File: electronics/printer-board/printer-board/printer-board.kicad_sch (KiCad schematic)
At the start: 38 parts, among them J1 XM, J10 THE1, J11 FAN1, J12 ZM1, J13 HE2, J14 THE2, J15 FAN2, J16 TFT, J17 EXP2, J18 EM0, J19 E0-Stop, J2 NeoPixel, J20 X-Stop, J21 EM1, J22 E1-Stop, J23 Y-Stop, J24 Bed, J25 I2C, J26 EM2, J27 E2-Stop, J28 Z-Stop, J29 Bed, J3 THB, J30 Hotend, J32 5V_PSU, J33 Hotend, J35 Extension1, J36 Extension2, J4 EXP1, J5 YM, J6 THE0, J7 FAN0, J8 BLTouch, J9 HE1

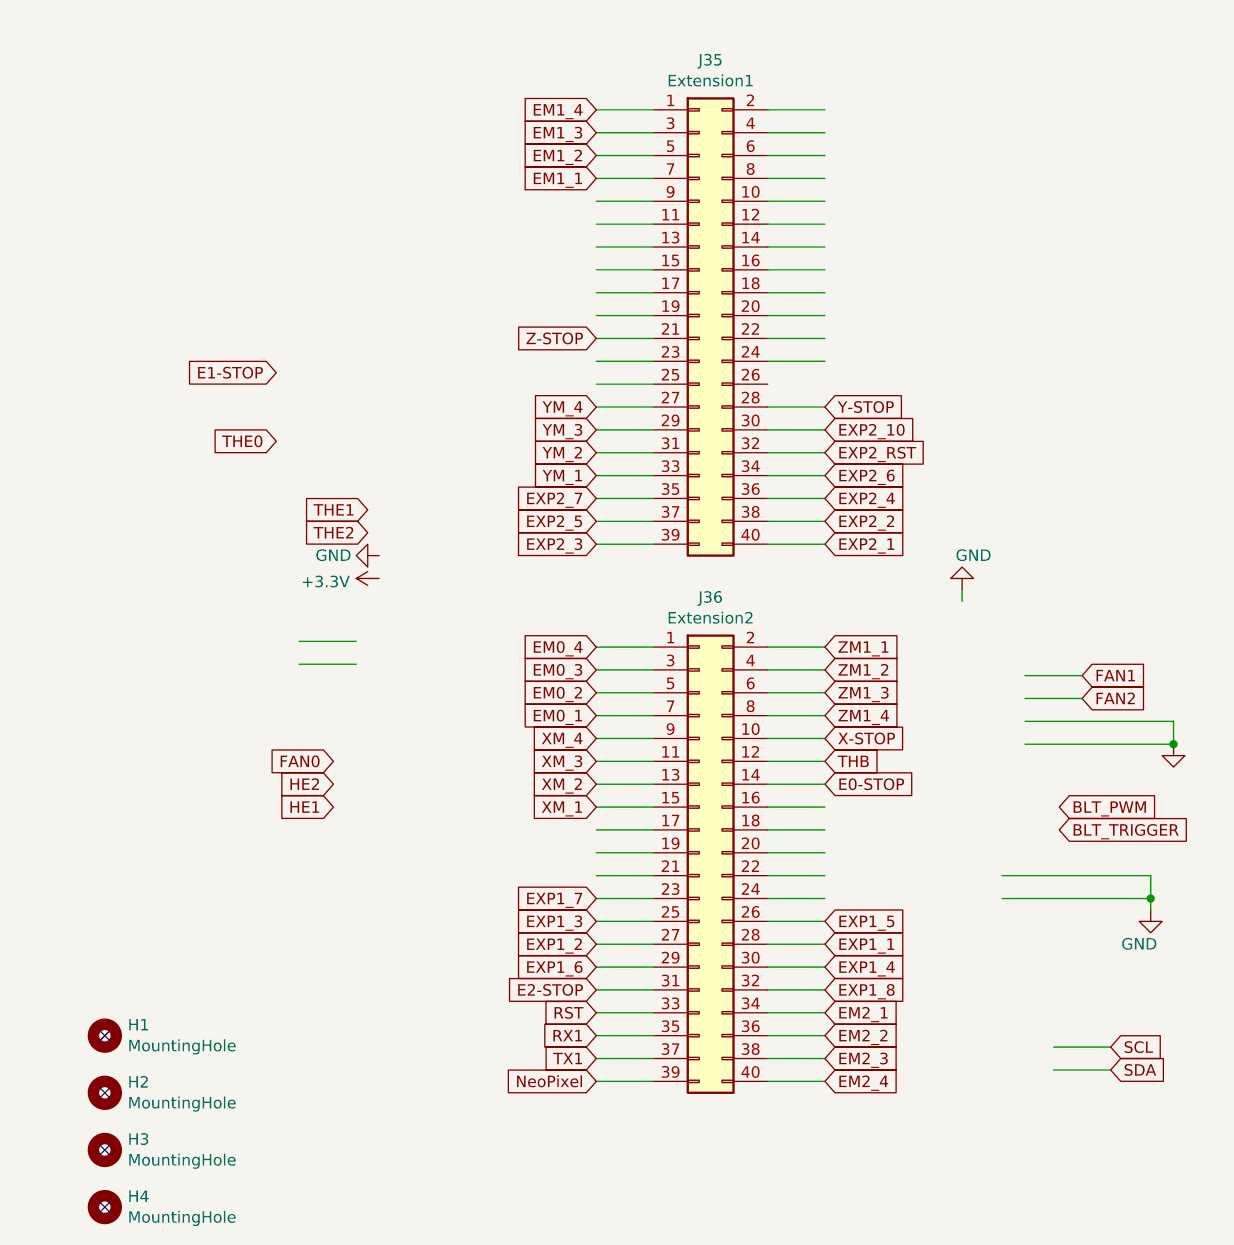
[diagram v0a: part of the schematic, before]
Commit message: updated routing
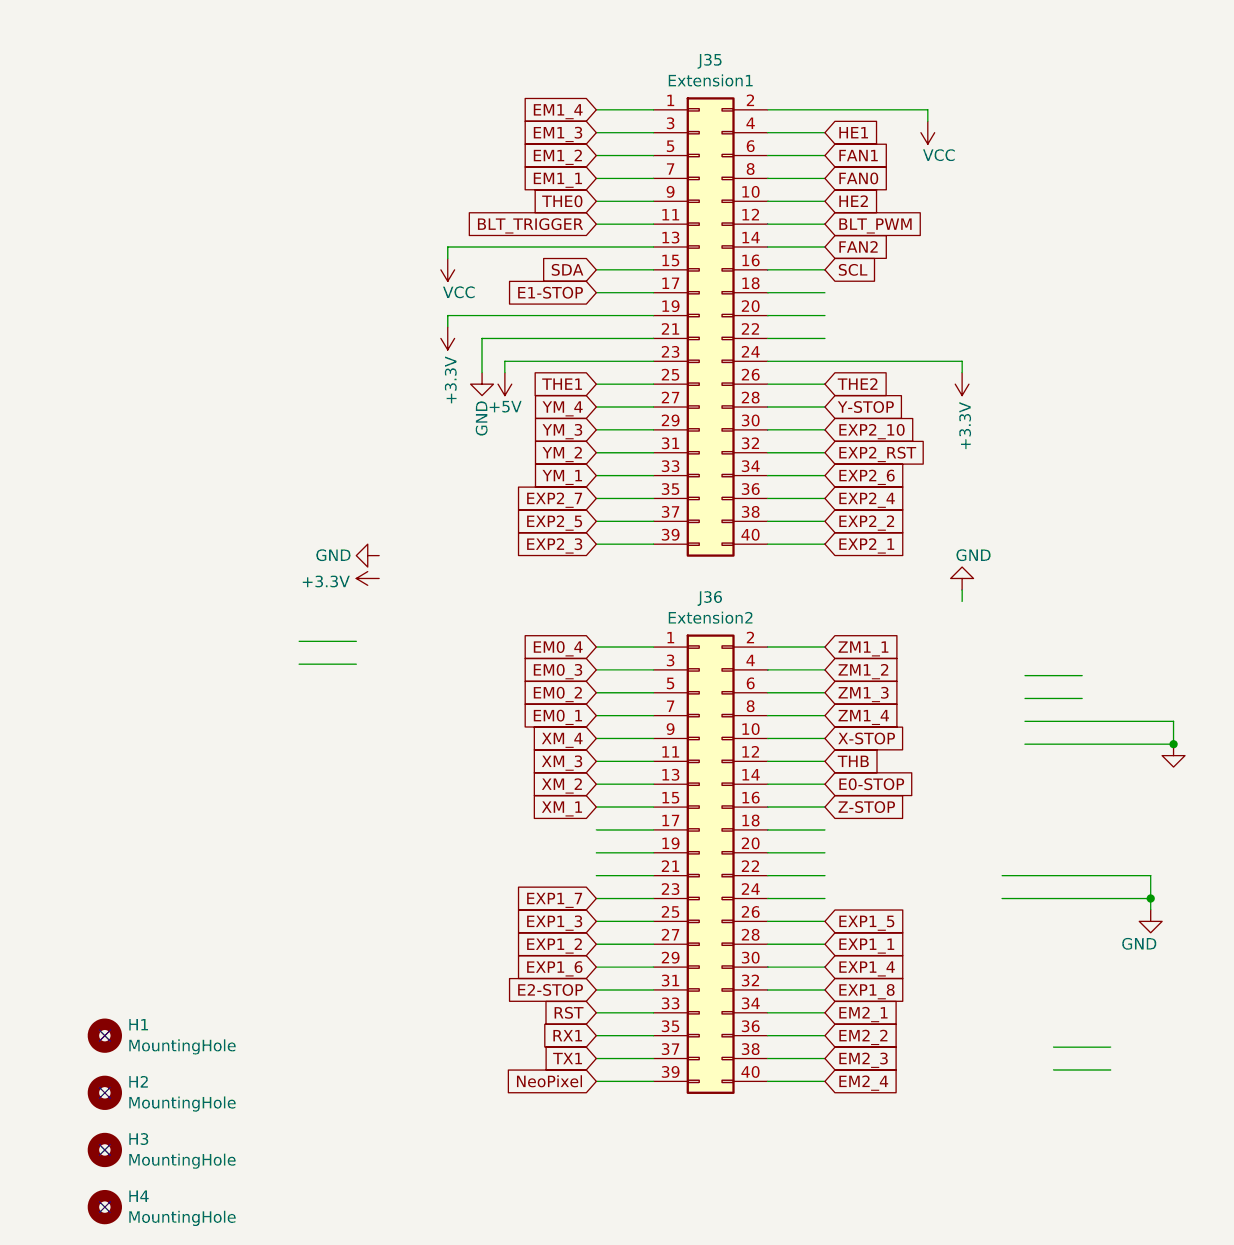
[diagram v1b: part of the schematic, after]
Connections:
- net +3V3: now also J35.19 (Pin_19), J35.24 (Pin_24)
- net +5V: now also J35.23 (Pin_23)
- net BLT_PWM: now also J35.12 (Pin_12)
- net BLT_TRIGGER: now also J35.11 (Pin_11)
- net E1-STOP: now also J35.17 (Pin_17)
- net FAN0: now also J35.8 (Pin_8)
- net FAN1: now also J35.6 (Pin_6)
- net FAN2: now also J35.14 (Pin_14)
- net GND: now also J35.21 (Pin_21)
- net HE1: now also J35.4 (Pin_4)
- net HE2: now also J35.10 (Pin_10)
- net SCL: now also J35.16 (Pin_16)
- net SDA: now also J35.15 (Pin_15)
- net THE0: now also J35.9 (Pin_9)
- net THE1: now also J35.25 (Pin_25)
- net THE2: now also J35.26 (Pin_26)
- net VCC: now also J35.13 (Pin_13), J35.2 (Pin_2)
- net Z-STOP: now also J36.16 (Pin_16); no longer J35.21 (Pin_21)
